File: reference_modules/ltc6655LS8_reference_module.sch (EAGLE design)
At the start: 8 parts

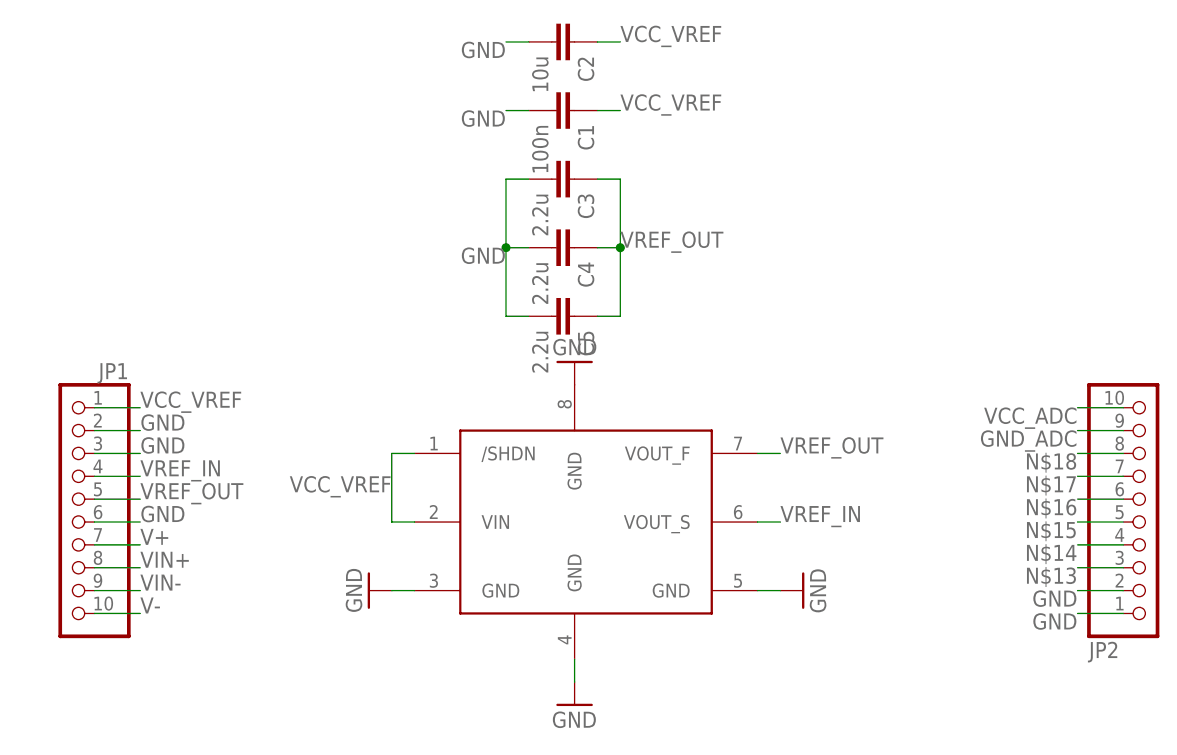
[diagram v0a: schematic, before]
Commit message: * finished ltc6655 reference board
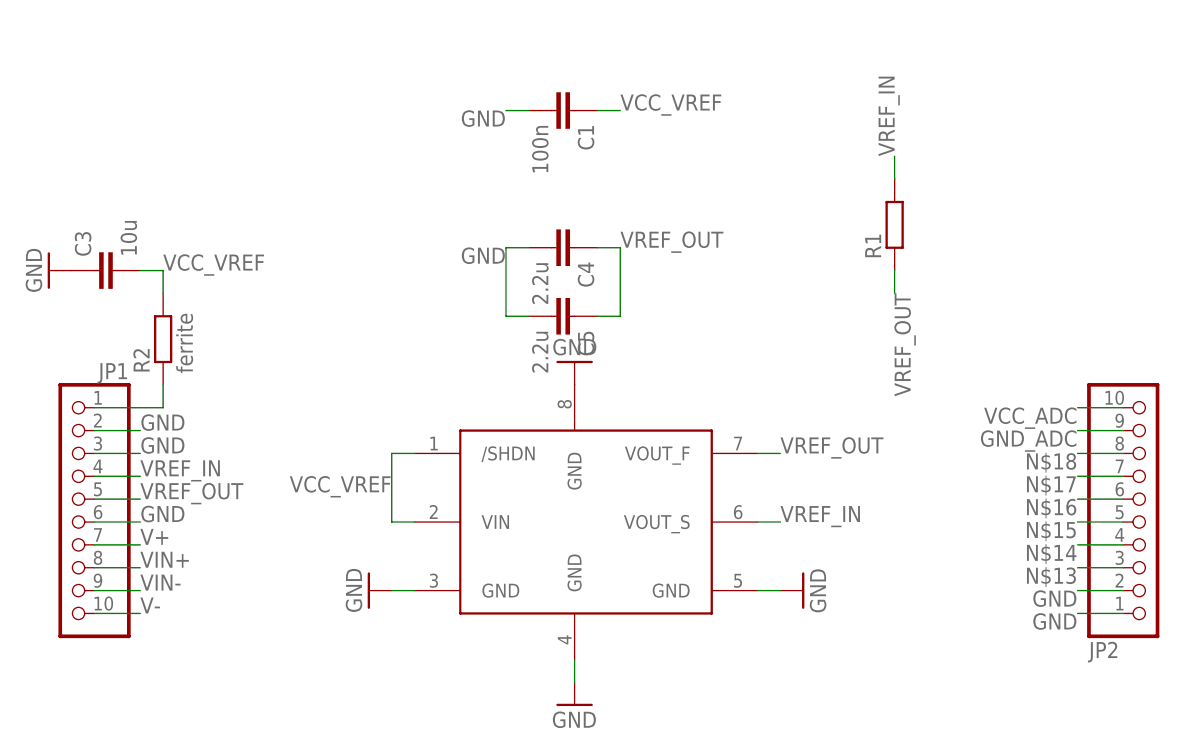
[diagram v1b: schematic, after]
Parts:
- removed C2: 10u, SquantorRCL:C-EUC0805
- added R1: (no value), SquantorRCL:R-EU_R1206
- added R2: ferrite, SquantorRCL:R-EU_R0805
- C3: value 2.2u -> 10u; device SquantorRCL:C-EUC2824W -> SquantorRCL:C-EUC0805
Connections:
- new net N$1: JP1.1, R2.1
- net GND: now also C3.1; no longer C2.2, C3.2
- net VCC_VREF: now also C3.2, R2.2; no longer C2.1, JP1.1
- net VREF_IN: now also R1.2
- net VREF_OUT: now also R1.1; no longer C3.1
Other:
- moved on the sheet: C3
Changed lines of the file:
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@@
 <layer number="115" name="ReferenceISLANDS" color="7" fill="1" visible="yes" active="yes"/>
 <layer number="116" name="Patch_BOT" color="9" fill="4" visible="yes" active="yes"/>
+<layer number="117" name="BACKMAAT1" color="7" fill="1" visible="yes" active="yes"/>
 <layer number="118" name="Rect_Pads" color="7" fill="1" visible="yes" active="yes"/>
+<layer number="119" name="KAP_TEKEN" color="7" fill="1" visible="yes" active="yes"/>
+<layer number="120" name="KAP_MAAT1" color="7" fill="1" visible="yes" active="yes"/>
 <layer number="121" name="_tsilk" color="7" fill="1" visible="yes" active="yes"/>
 <layer number="122" name="_bsilk" color="7" fill="1" visible="yes" active="yes"/>
@@
 <layer number="128" name="_bValues" color="7" fill="1" visible="yes" active="yes"/>
 <layer number="129" name="Mask" color="7" fill="1" visible="yes" active="yes"/>
+<layer number="130" name="SMDSTROOK" color="7" fill="1" visible="yes" active="yes"/>
 <layer number="131" name="tAdjust" color="7" fill="1" visible="yes" active="yes"/>
 <layer number="132" name="bAdjust" color="7" fill="1" visible="yes" active="yes"/>
+<layer number="133" name="BGA_CORE_SUP" color="12" fill="1" visible="yes" active="yes"/>
+<layer number="134" name="BGA_GND" color="1" fill="1" visible="yes" active="yes"/>
+<layer number="135" name="BGA_NC" color="8" fill="1" visible="yes" active="yes"/>
+<layer number="136" name="BGA_DED" color="14" fill="1" visible="yes" active="yes"/>
 <layer number="144" name="Drill_legend" color="7" fill="1" visible="yes" active="yes"/>
 <layer number="150" name="Notes" color="7" fill="1" visible="yes" active="yes"/>
@@
 <part name="JP2" library="SquantorConnectors" deviceset="PINHD-1X10" device="NORM_OCT"/>
 <part name="U$1" library="SquantorLinearTechnology" deviceset="LTC6655" device="LS8_ELONG"/>
-<part name="C2" library="SquantorRCL" deviceset="C-EU" device="C0805" value="10u"/>
 <part name="C1" library="SquantorRCL" deviceset="C-EU" device="C0603" value="100n"/>
-<part name="C3" library="SquantorRCL" deviceset="C-EU" device="C2824W" value="2.2u"/>
 <part name="C4" library="SquantorRCL" deviceset="C-EU" device="C2824W" value="2.2u"/>
 <part name="C5" library="SquantorRCL" deviceset="C-EU" device="C2824W" value="2.2u"/>
@@
 <part name="GND3" library="supply1" deviceset="GND" device=""/>
 <part name="GND4" library="supply1" deviceset="GND" device=""/>
+<part name="R1" library="SquantorRCL" deviceset="R-EU_" device="R1206"/>
+<part name="R2" library="SquantorRCL" deviceset="R-EU_" device="R0805" value="ferrite"/>
+<part name="C3" library="SquantorRCL" deviceset="C-EU" device="C0805" value="10u"/>
+<part name="GND5" library="supply1" deviceset="GND" device=""/>
 </parts>
 <sheets>
@@
 <instance part="JP2" gate="A" x="134.62" y="30.48" rot="MR180"/>
 <instance part="U$1" gate="G$1" x="71.12" y="27.94"/>
-<instance part="C2" gate="G$1" x="71.12" y="83.82" rot="R270"/>
 <instance part="C1" gate="G$1" x="71.12" y="76.2" rot="R270"/>
-<instance part="C3" gate="G$1" x="71.12" y="68.58" rot="R270"/>
 <instance part="C4" gate="G$1" x="71.12" y="60.96" rot="R270"/>
 <instance part="C5" gate="G$1" x="71.12" y="53.34" rot="R270"/>
@@
 <instance part="GND3" gate="1" x="48.26" y="22.86" rot="R270"/>
 <instance part="GND4" gate="1" x="71.12" y="48.26" rot="R180"/>
+<instance part="R1" gate="G$1" x="106.68" y="63.5" rot="R90"/>
+<instance part="R2" gate="G$1" x="25.4" y="50.8" rot="R90"/>
+<instance part="C3" gate="G$1" x="17.78" y="58.42" rot="R90"/>
+<instance part="GND5" gate="1" x="12.7" y="58.42" rot="R270"/>
 </instances>
 <busses>
@@
 <nets>
 <net name="VCC_VREF" class="0">
-<segment>
-<pinref part="JP1" gate="A" pin="1"/>
-<wire x1="17.78" y1="43.18" x2="22.86" y2="43.18" width="0.1524" layer="91"/>
-<label x="22.86" y="43.18" size="1.778" layer="95"/>
-</segment>
-<segment>
-<pinref part="C2" gate="G$1" pin="1"/>
-<wire x1="73.66" y1="83.82" x2="76.2" y2="83.82" width="0.1524" layer="91"/>
-<label x="76.2" y="83.82" size="1.778" layer="95"/>
-</segment>
 <segment>
 <pinref part="C1" gate="G$1" pin="1"/>
@@
 <label x="50.8" y="35.56" size="1.778" layer="95" rot="R180"/>
 </segment>
+<segment>
+<pinref part="R2" gate="G$1" pin="2"/>
+<wire x1="25.4" y1="55.88" x2="25.4" y2="58.42" width="0.1524" layer="91"/>
+<pinref part="C3" gate="G$1" pin="2"/>
+<wire x1="25.4" y1="58.42" x2="22.86" y2="58.42" width="0.1524" layer="91"/>
+<label x="25.4" y="58.42" size="1.778" layer="95"/>
+</segment>
 </net>
 <net name="VREF_IN" class="0">
@@
 <label x="93.98" y="30.48" size="1.778" layer="95"/>
 </segment>
+<segment>
+<pinref part="R1" gate="G$1" pin="2"/>
+<wire x1="106.68" y1="68.58" x2="106.68" y2="71.12" width="0.1524" layer="91"/>
+<label x="106.68" y="71.12" size="1.778" layer="95" rot="R90"/>
+</segment>
 </net>
 <net name="VREF_OUT" class="0">
@@
 </segment>
 <segment>
-<pinref part="C3" gate="G$1" pin="1"/>
-<wire x1="73.66" y1="68.58" x2="76.2" y2="68.58" width="0.1524" layer="91"/>
-<wire x1="76.2" y1="68.58" x2="76.2" y2="60.96" width="0.1524" layer="91"/>
 <pinref part="C5" gate="G$1" pin="1"/>
 <wire x1="76.2" y1="60.96" x2="76.2" y2="53.34" width="0.1524" layer="91"/>
@@
 <pinref part="C4" gate="G$1" pin="1"/>
 <wire x1="73.66" y1="60.96" x2="76.2" y2="60.96" width="0.1524" layer="91"/>
-<junction x="76.2" y="60.96"/>
 <label x="76.2" y="60.96" size="1.778" layer="95"/>
+</segment>
+<segment>
+<pinref part="R1" gate="G$1" pin="1"/>
+<wire x1="106.68" y1="58.42" x2="106.68" y2="55.88" width="0.1524" layer="91"/>
+<label x="106.68" y="55.88" size="1.778" layer="95" rot="R270"/>
 </segment>
 </net>
@@
 </segment>
 <segment>
-<pinref part="C3" gate="G$1" pin="2"/>
-<wire x1="66.04" y1="68.58" x2="63.5" y2="68.58" width="0.1524" layer="91"/>
-<wire x1="63.5" y1="68.58" x2="63.5" y2="60.96" width="0.1524" layer="91"/>
 <pinref part="C5" gate="G$1" pin="2"/>
 <wire x1="63.5" y1="60.96" x2="63.5" y2="53.34" width="0.1524" layer="91"/>
@@
 <pinref part="C4" gate="G$1" pin="2"/>
 <wire x1="63.5" y1="60.96" x2="66.04" y2="60.96" width="0.1524" layer="91"/>
-<junction x="63.5" y="60.96"/>
 <label x="63.5" y="60.96" size="1.778" layer="95" rot="R180"/>
 </segment>
@@
 </segment>
 <segment>
-<pinref part="C2" gate="G$1" pin="2"/>
-<wire x1="66.04" y1="83.82" x2="63.5" y2="83.82" width="0.1524" layer="91"/>
-<label x="63.5" y="83.82" size="1.778" layer="95" rot="R180"/>
+<pinref part="C3" gate="G$1" pin="1"/>
+<pinref part="GND5" gate="1" pin="GND"/>
 </segment>
 </net>
@@
 </segment>
 </net>
+<net name="N$1" class="0">
+<segment>
+<pinref part="JP1" gate="A" pin="1"/>
+<wire x1="17.78" y1="43.18" x2="25.4" y2="43.18" width="0.1524" layer="91"/>
+<pinref part="R2" gate="G$1" pin="1"/>
+<wire x1="25.4" y1="43.18" x2="25.4" y2="45.72" width="0.1524" layer="91"/>
+</segment>
+</net>
